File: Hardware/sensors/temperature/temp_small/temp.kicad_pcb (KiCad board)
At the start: 2 copper layers, 20.6 x 4.6 mm, 7 parts, among them J1 Conn_01x01, J2 Conn_01x01, J3 Conn_01x01, J4 Conn_01x01, J5 Conn_01x01, J6 Conn_01x01, U1 TMP1826DGK

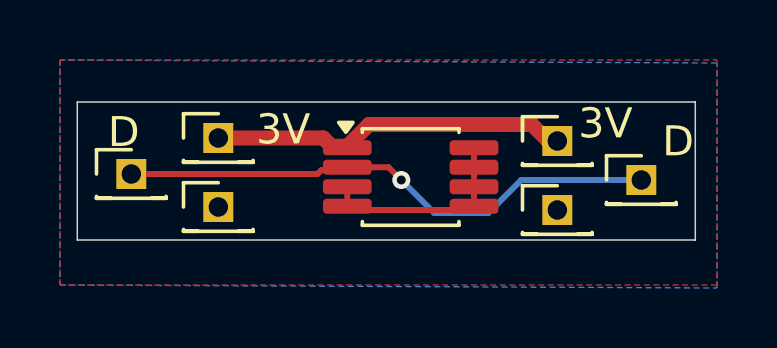
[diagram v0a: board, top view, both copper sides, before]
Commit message: Corrected errors in PCB
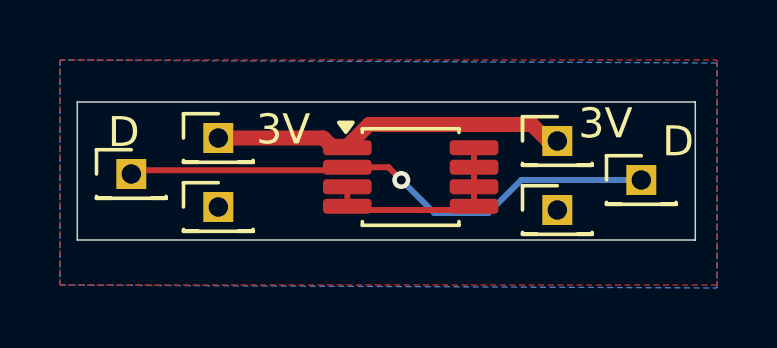
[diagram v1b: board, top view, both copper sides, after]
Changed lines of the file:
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@@
 			(outputformat 1)
 			(mirror no)
-			(drillshape 1)
+			(drillshape 0)
 			(scaleselection 1)
-			(outputdirectory "")
+			(outputdirectory "/home/cornut/Documents/datalogger/Hardware/sensors/temperature/temp_small/")
 		)
 	)
@@
 	)
 	(segment
+		(start 125.325 81.375)
+		(end 125.2 81.5)
+		(width 0.2)
+		(layer "F.Cu")
+		(net 3)
+	)
+	(segment
 		(start 134.075 81.275)
 		(end 132.7 81.275)
@@
 	)
 	(segment
-		(start 131.832994 81.375)
-		(end 131.707994 81.5)
-		(width 0.2)
-		(layer "F.Cu")
-		(net 3)
-	)
-	(segment
-		(start 131.707994 81.5)
-		(end 125.2 81.5)
-		(width 0.2)
-		(layer "F.Cu")
-		(net 3)
-	)
-	(segment
 		(start 132.7 81.275)
 		(end 132.6 81.375)
@@
 	)
 	(segment
+		(start 132.6 81.375)
+		(end 125.325 81.375)
+		(width 0.2)
+		(layer "F.Cu")
+		(net 3)
+	)
+	(segment
 		(start 134.5 81.7)
 		(end 134.075 81.275)
 		(width 0.2)
 		(layer "F.Cu")
-		(net 3)
-	)
-	(segment
-		(start 132.6 81.375)
-		(end 131.832994 81.375)
-		(width 0.2)
-		(layer "F.Cu")
